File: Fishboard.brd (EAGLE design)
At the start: 47.9 x 61 mm, 23 parts, among them J3 B1, J4 B2, J5 B3, J7 B4, Q1 TIP120, Q2 TIP120, Q3 TIP120

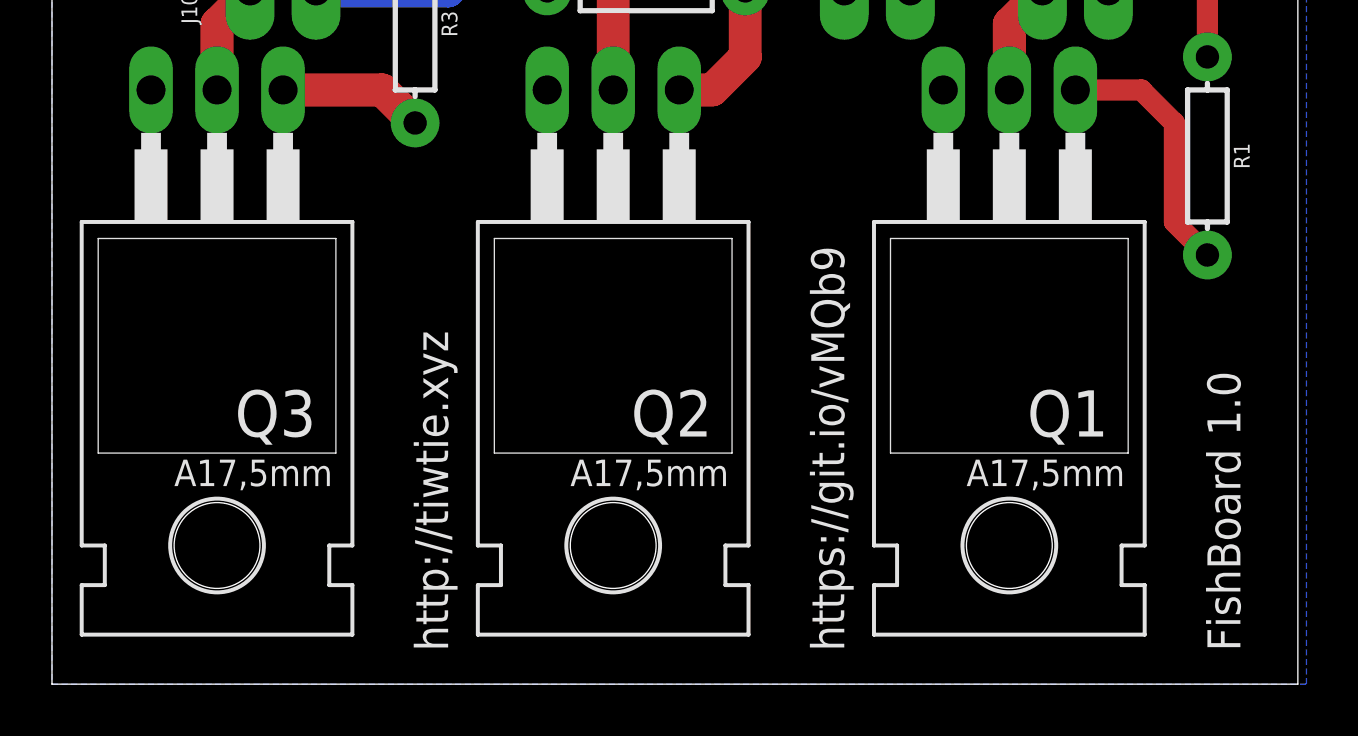
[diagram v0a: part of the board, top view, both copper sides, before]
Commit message: Reorganized schematics
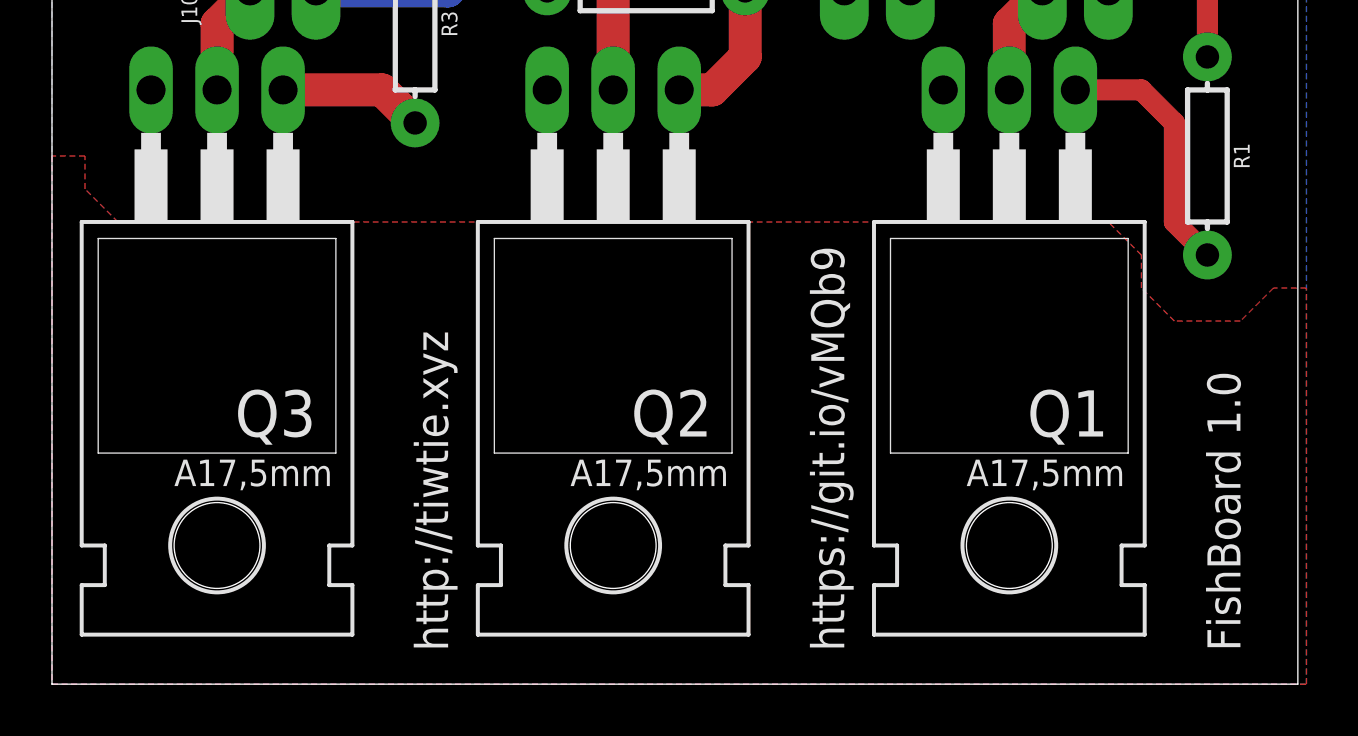
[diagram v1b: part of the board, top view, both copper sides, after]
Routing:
- added copper zone on layer 1, net N$7
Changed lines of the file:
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@@
 <wire x1="30.48" y1="27.94" x2="30.48" y2="26.67" width="1.27" layer="1"/>
+</signal>
+<signal name="N$7">
+<polygon width="0.4064" layer="1">
+<vertex x="1.27" y="20.32"/>
+<vertex x="0" y="20.32"/>
+<vertex x="0" y="0"/>
+<vertex x="48.26" y="0"/>
+<vertex x="48.26" y="15.24"/>
+<vertex x="46.99" y="15.24"/>
+<vertex x="45.72" y="13.97"/>
+<vertex x="43.18" y="13.97"/>
+<vertex x="41.91" y="15.24"/>
+<vertex x="41.91" y="16.51"/>
+<vertex x="40.64" y="17.78"/>
+<vertex x="2.54" y="17.78"/>
+<vertex x="1.27" y="19.05"/>
+</polygon>
 </signal>
 </signals>
